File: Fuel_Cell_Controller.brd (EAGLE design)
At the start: 203.2 x 163.8 mm, 130 parts, among them J1 BLUETOOTH, U1 MAX232PTH

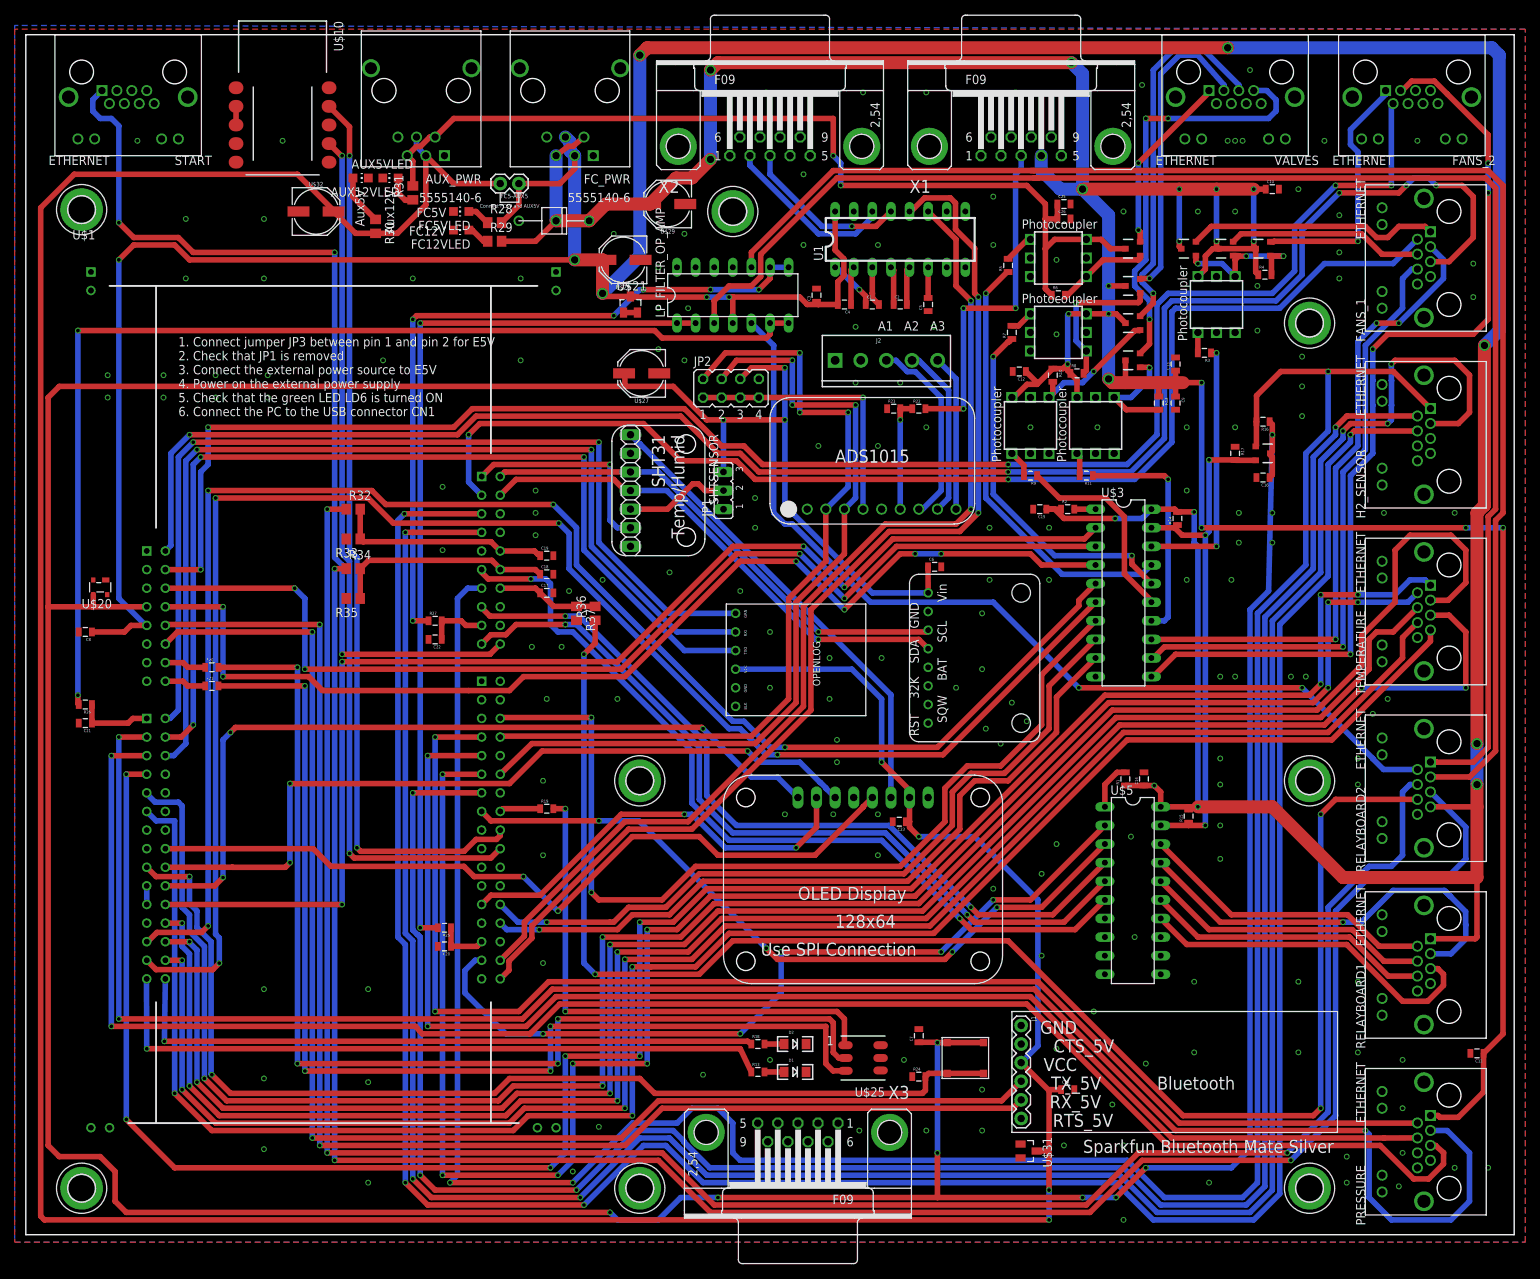
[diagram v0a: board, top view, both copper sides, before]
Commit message: Some Updates
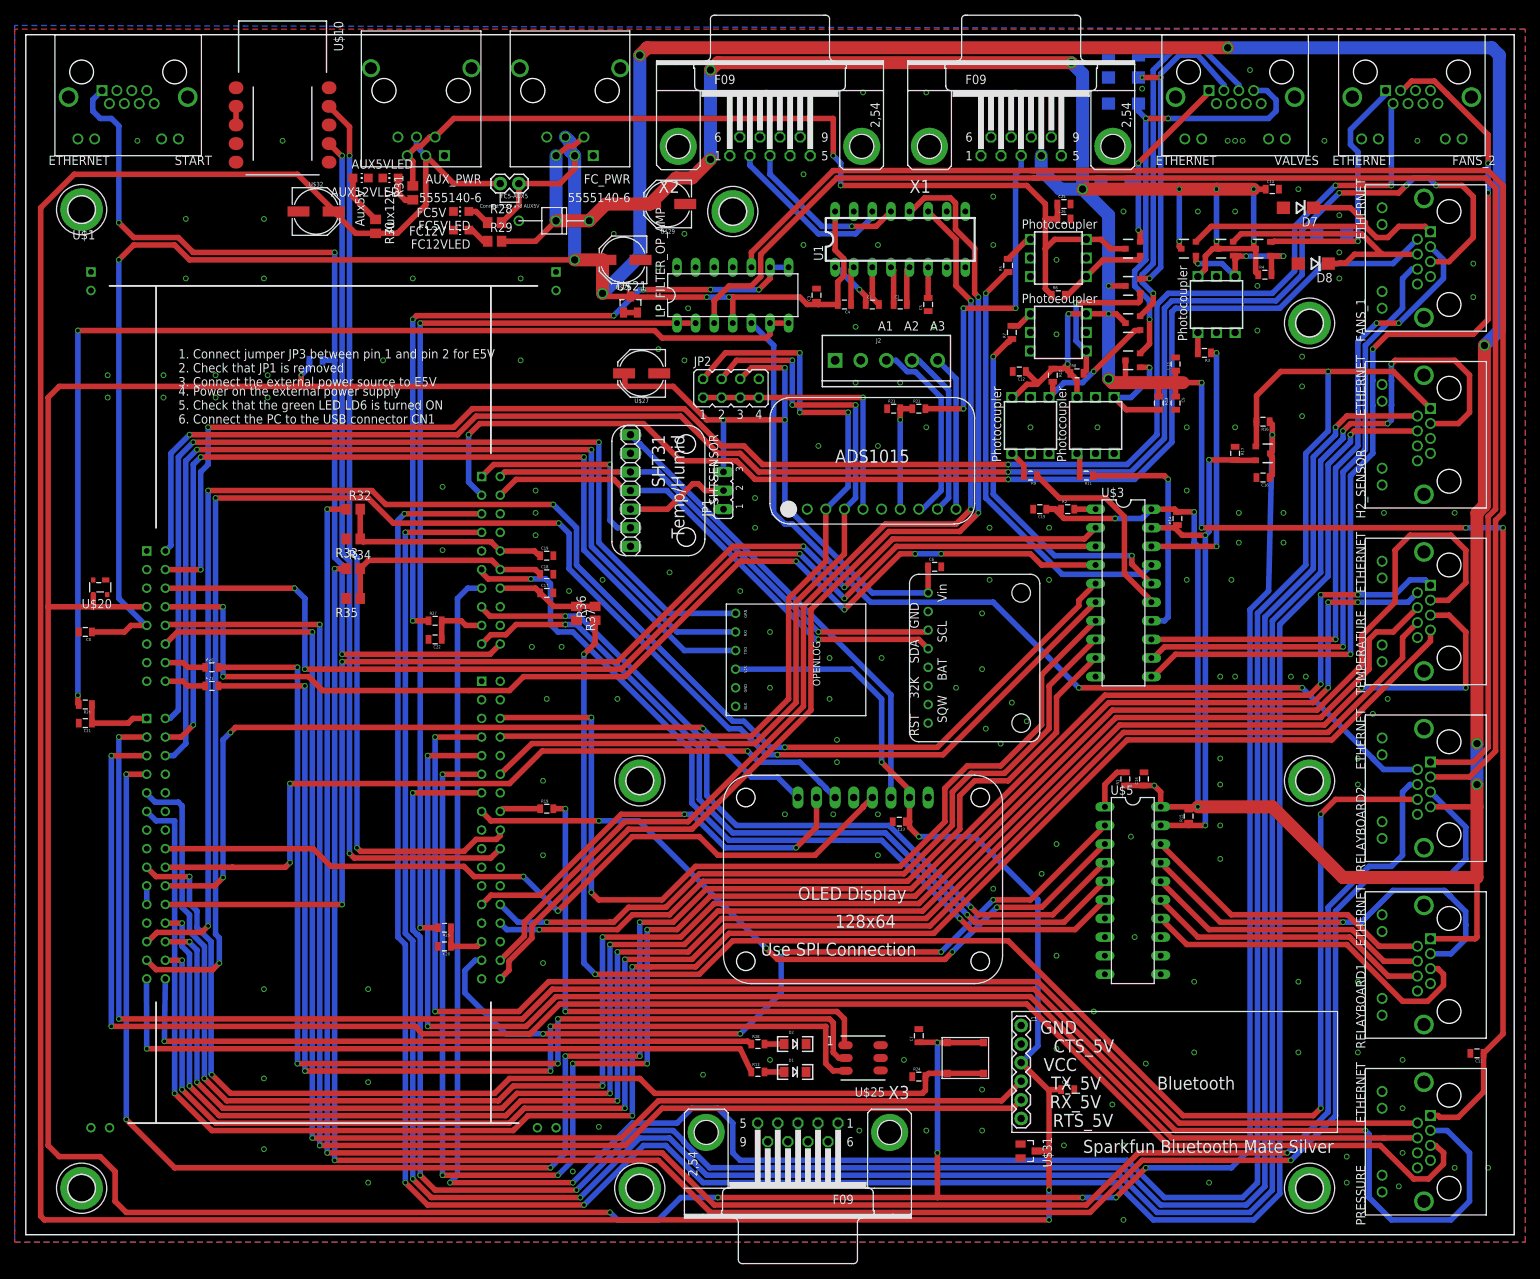
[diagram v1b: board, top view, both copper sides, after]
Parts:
- added D3, D4, D5, D6, D7, D8, D9: (no value), diode:DO214AC
- added R38: 1kΩ, SparkFun-Passives:0805
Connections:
- net FAN1_PWR: now also D7.C
- net FAN2_PWR: now also D8.C
- net FAN3_PWR: now also D9.C
- net GND: now also D3.A, D4.A, D5.A, D6.A, D7.A, D8.A, D9.A
- net NUC_3V3: now also R38.2
- net OUTPUT_1_ENET: now also D5.C
- net OUTPUT_2_ENET: now also D3.C
- net PURGE_VALVE_ENET: now also D6.C
- net SUPPLY_VALVE_ENET: now also D4.C
- net _START: now also R38.1
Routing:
- net FAN1_PWR: track 34.5 -> 42.9 mm
- net FAN2_PWR: track 26.8 -> 34.6 mm
- net NUC_3V3: track 594.4 -> 598.5 mm, vias 11 -> 12
- net OUTPUT_1_ENET: track 51.4 -> 55.2 mm
- net PURGE_VALVE_ENET: track 42.2 -> 45.2 mm, vias 1 -> 3
- net OUTPUT_2_ENET: track 57.4 -> 59.8 mm
- net _START: track 129.5 -> 131.2 mm
- net FAN3_PWR: track 35.0 -> 36.5 mm
- net SUPPLY_VALVE_ENET: track 24.7 -> 25.7 mm
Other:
- board text added: "1. Connect jumper JP3 between pin 1 and pin 2 for E5V 2. Check that JP1 is removed 3. Connect the external power source to E5V"
- board text added: "4. Power on the external power supply 5. Check that the green LED LD6 is turned ON 6. Connect the PC to the USB connector CN1"
- board text removed: "1. Connect jumper JP3 between pin 1 and pin 2 for E5V 2. Check that JP1 is removed 3. Connect the external power source to E5V 4. Power on the external power supply 5. Check that the green LED LD6 is turned ON 6. Connect the PC to the USB connector CN1"
